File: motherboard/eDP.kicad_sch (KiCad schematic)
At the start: 2 parts, among them J2 20455-040E-76 OLED IPEX, J6 OLED EL POWER

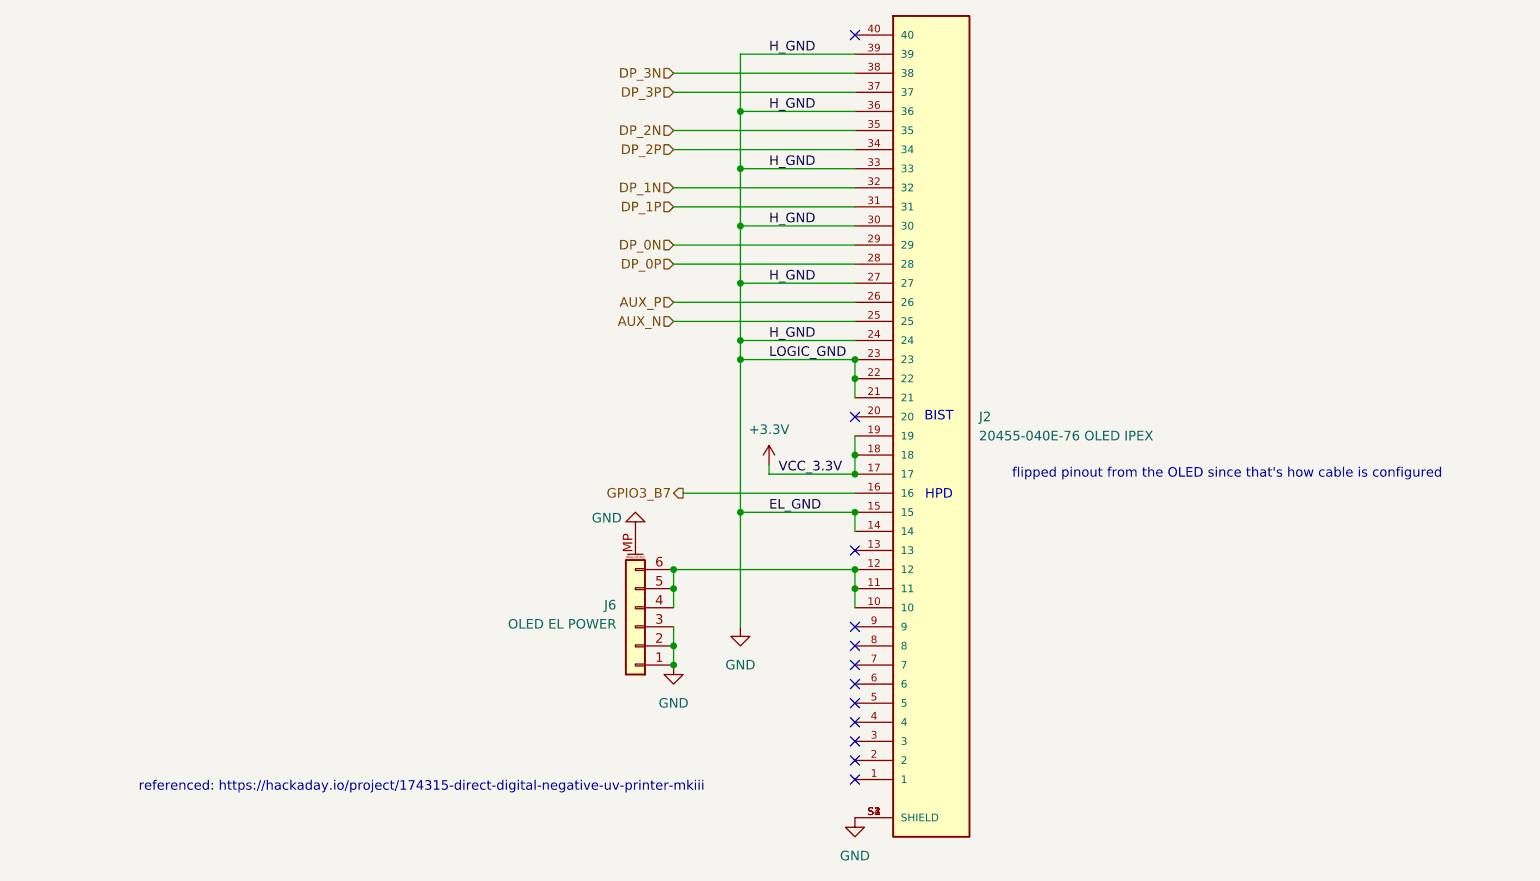
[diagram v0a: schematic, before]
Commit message: mainboard v0.3 + power WIP
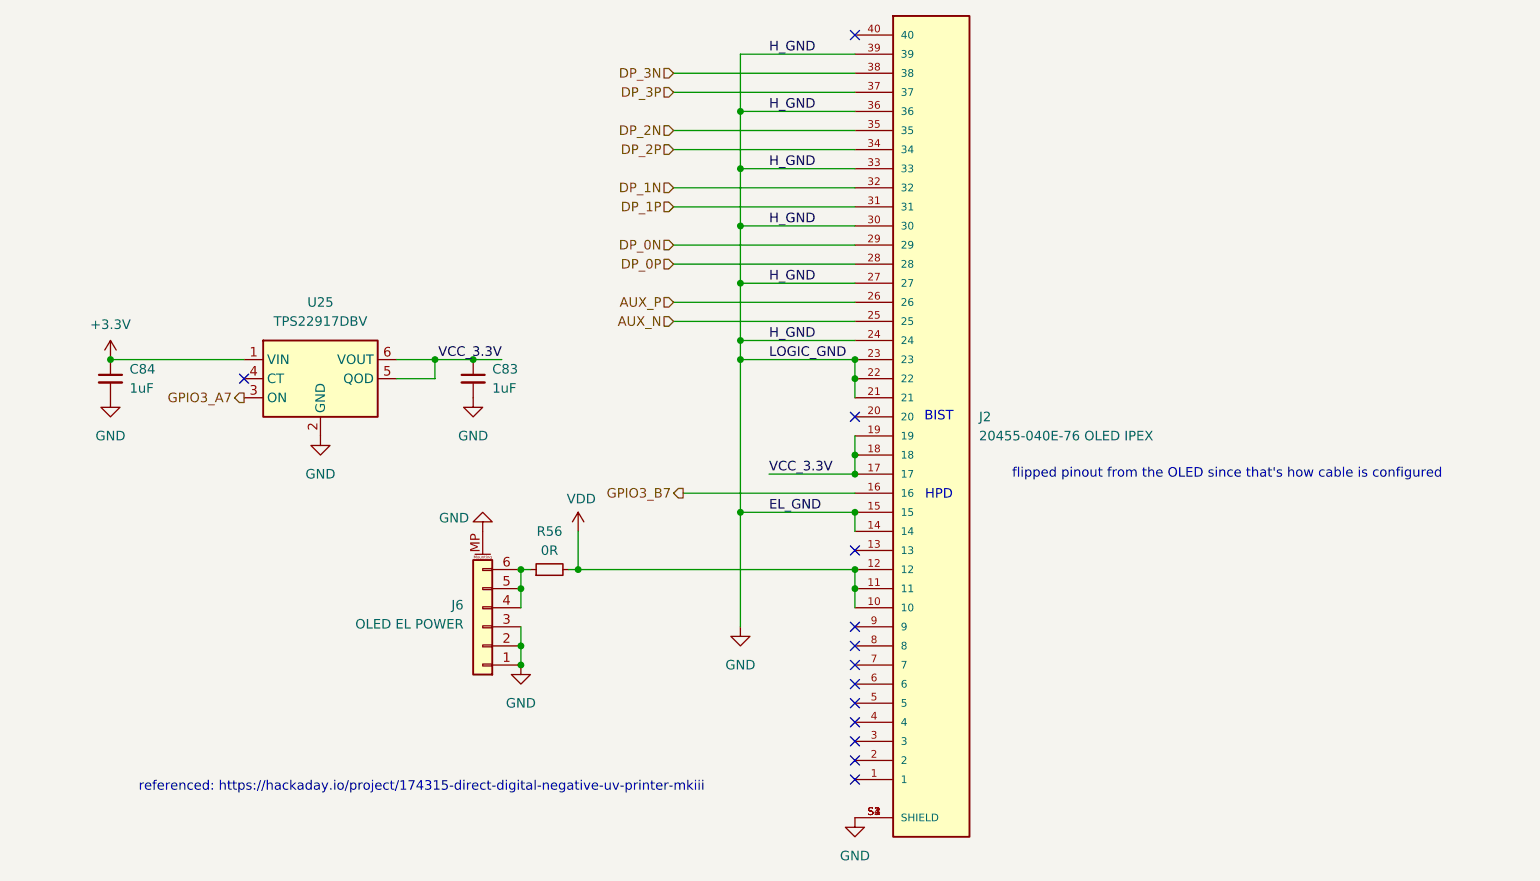
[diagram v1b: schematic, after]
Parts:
- added C83, C84: 1uF, Capacitor_SMD:C_0402_1005Metric, symbol Device:C_Small
- added R56: 0R, Jumper:SolderJumper-2_P1.3mm_Open_TrianglePad1.0x1.5mm, symbol Device:R_Small
- added U25: TPS22917DBV, Package_TO_SOT_SMD:SOT-23-6, symbol Power_Management:TPS22917DBV
- J2: footprint 20455-040E-76:IPEX_20455-040E-76 -> eDP_Connector:IPEX_20455-040E-76
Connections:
- net +3.3V: now also C84.1, U25.1 (VIN); no longer J2.17, J2.18, J2.19
- net GND: now also C83.2, C84.2, U25.2 (GND)
- net at J6.4 (Pin_4), J6.5 (Pin_5), J6.6 (Pin_6): now also R56.1; no longer J2.10, J2.11, J2.12
- new net GPIO3_A7: U25.3 (ON)
- new net VCC_3.3V: C83.1, J2.17, J2.18, J2.19, U25.5 (QOD), U25.6 (VOUT)
- new net VDD: J2.10, J2.11, J2.12, R56.2
- no-connect marks 12 -> 13
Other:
- moved on the sheet: J6
